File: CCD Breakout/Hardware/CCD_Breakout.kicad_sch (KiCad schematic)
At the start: 1 part

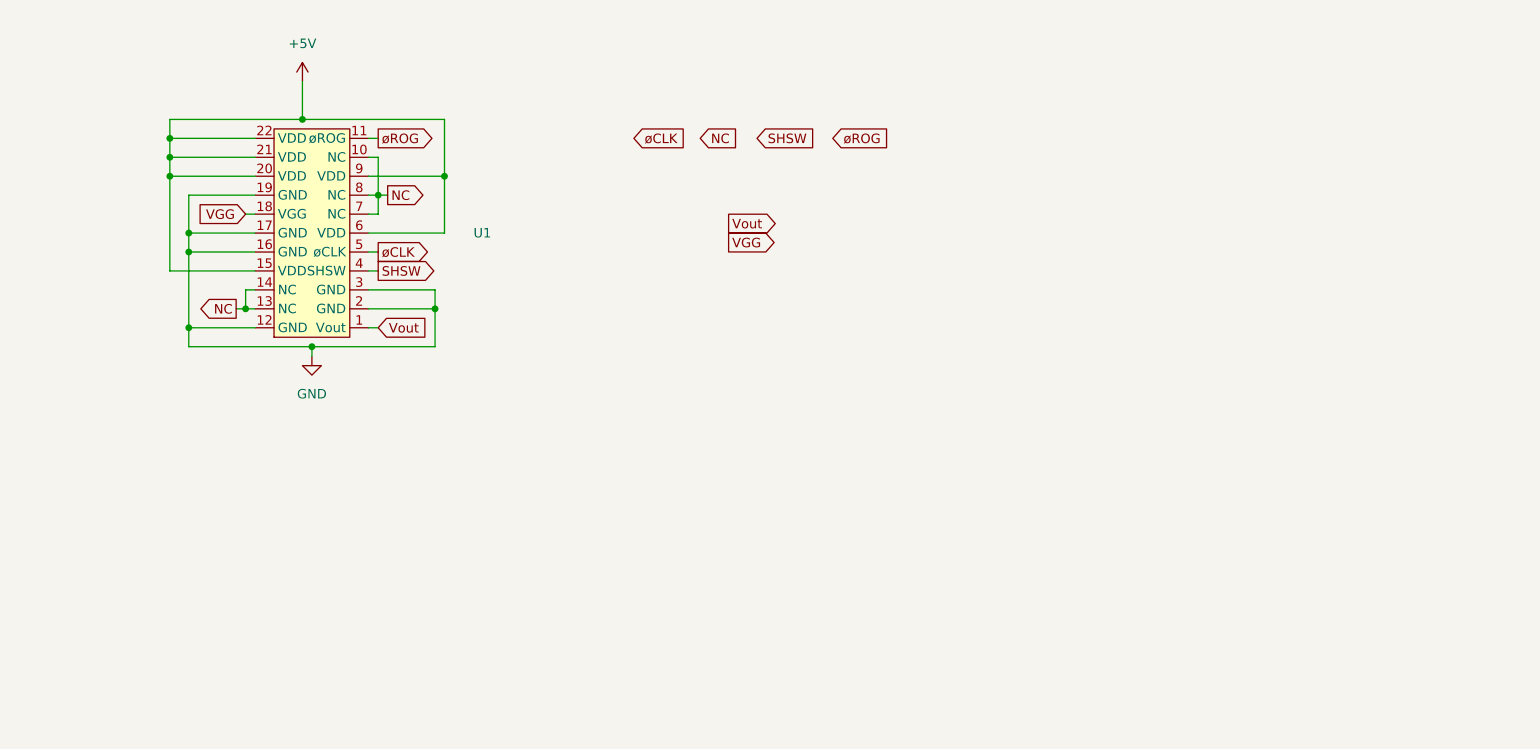
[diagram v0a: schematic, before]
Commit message: //WIP CCD Breakout
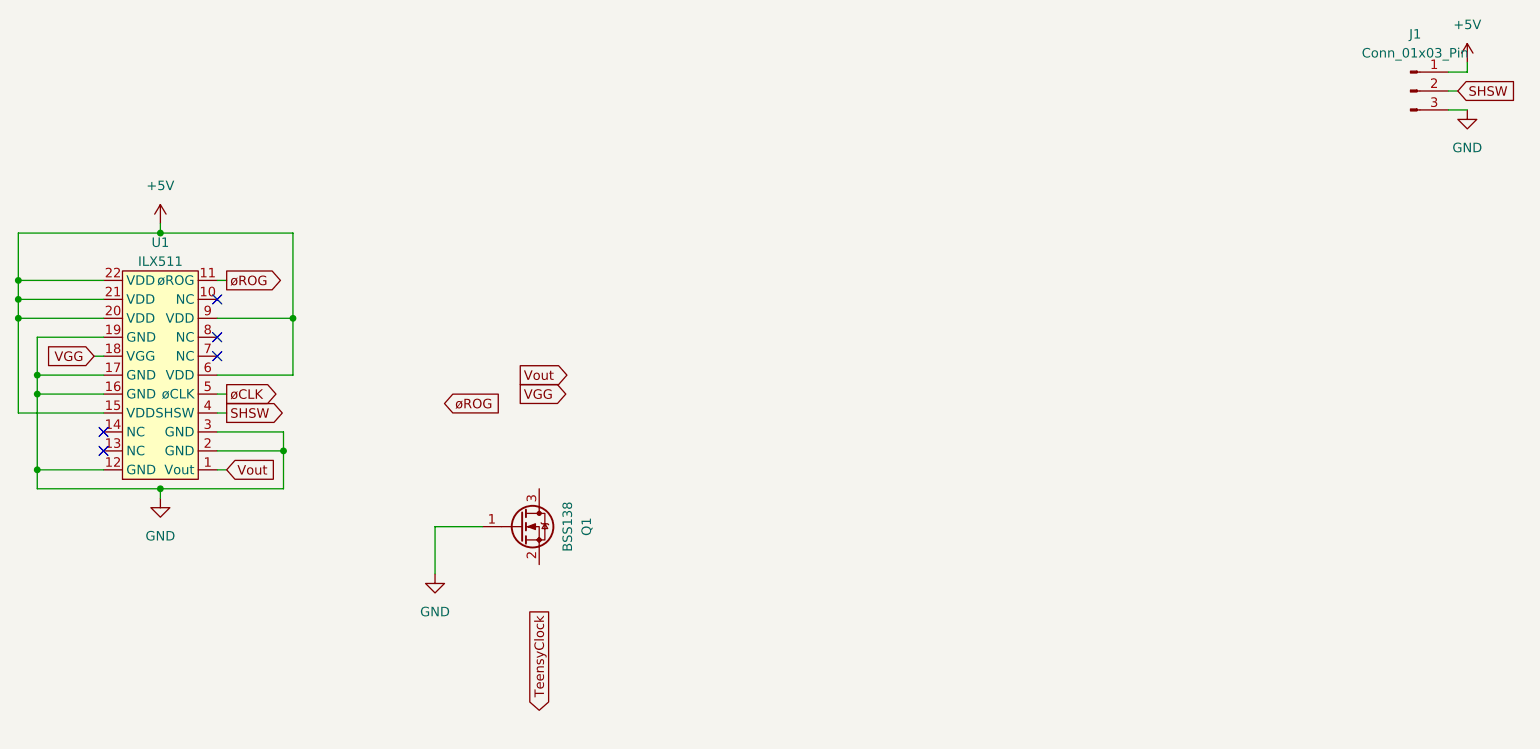
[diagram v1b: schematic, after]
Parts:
- added J1: Conn_01x03_Pin, symbol Connector:Conn_01x03_Pin
- added Q1: BSS138, Package_TO_SOT_SMD:SOT-23, symbol Transistor_FET:BSS138
- U1: value ~ -> ILX511
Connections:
- net +5V: now also J1.1 (Pin_1)
- net GND: now also J1.3 (Pin_3), Q1.1 (G)
- net SHSW: now also J1.2 (Pin_2)
- removed net NC: U1.10 (NC), U1.13 (NC), U1.14 (NC), U1.7 (NC), U1.8 (NC)
- no-connect marks 0 -> 5
